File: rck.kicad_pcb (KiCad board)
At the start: 2 copper layers, 142.3 x 183.9 mm, 40 parts, among them J01 Conn_02x22_Row_Letter_Last, J02 Conn_02x22_Row_Letter_Last, J03 Conn_02x22_Row_Letter_Last, J04 Conn_02x22_Row_Letter_Last

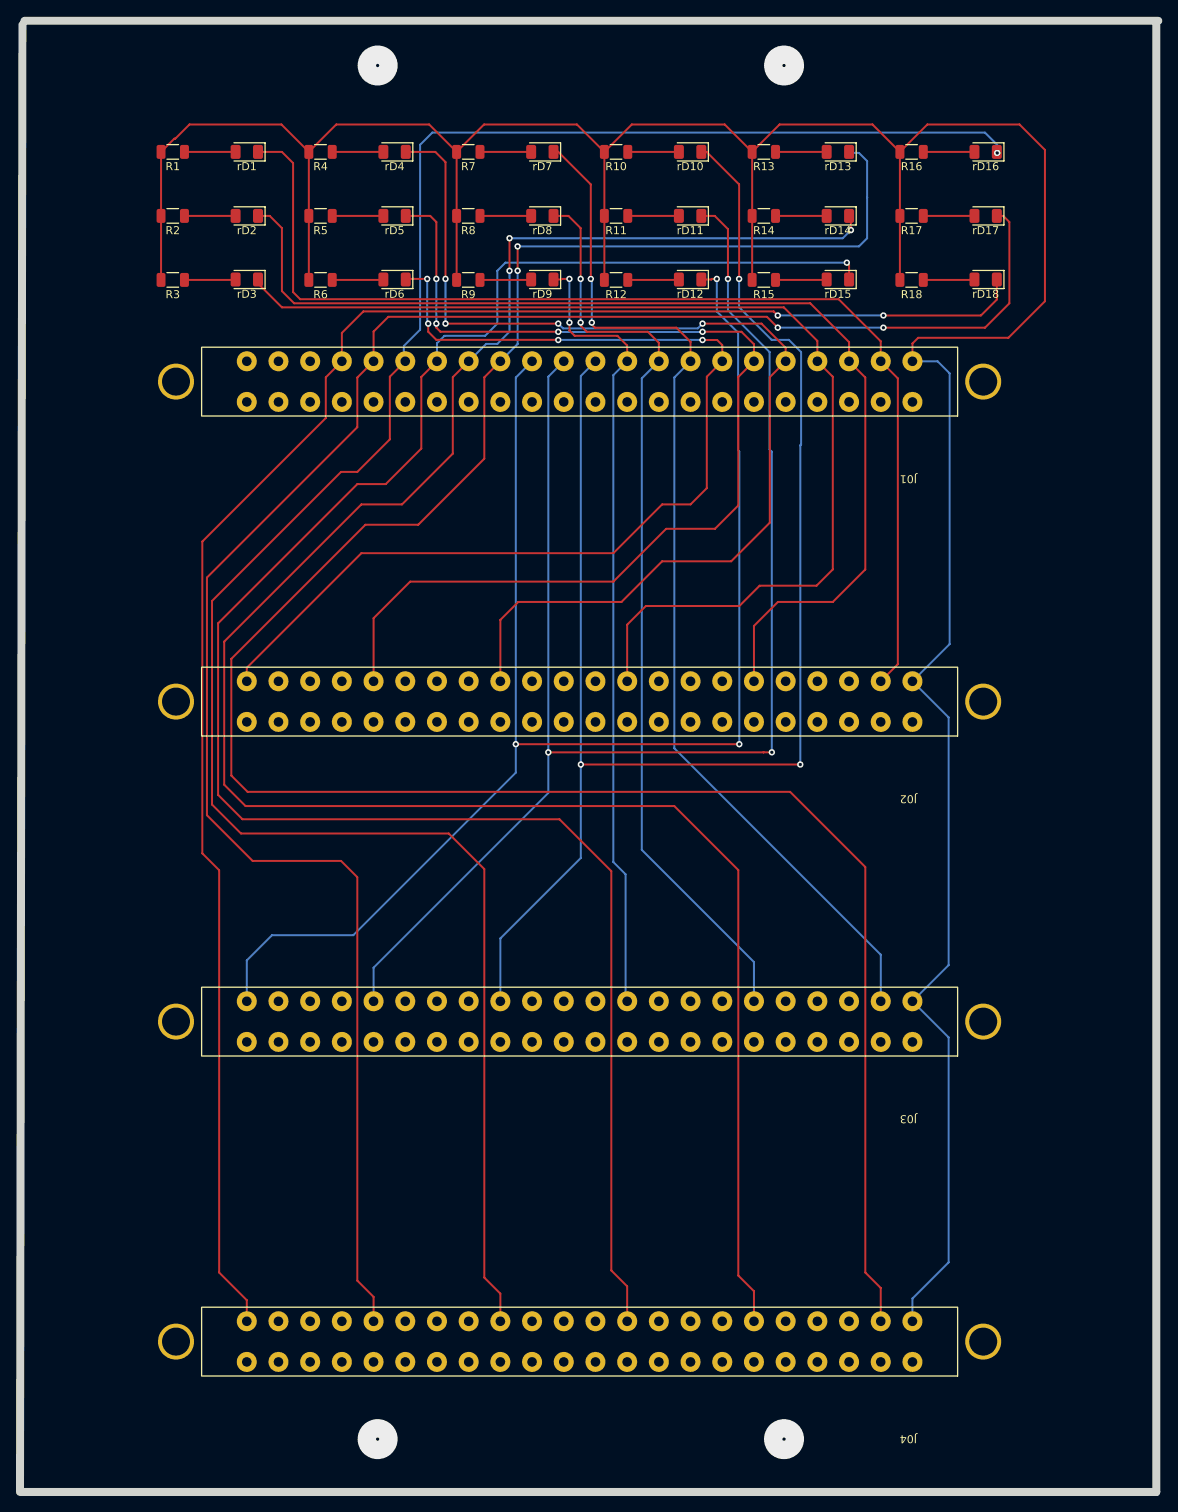
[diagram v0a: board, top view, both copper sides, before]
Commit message: V1.0Rack
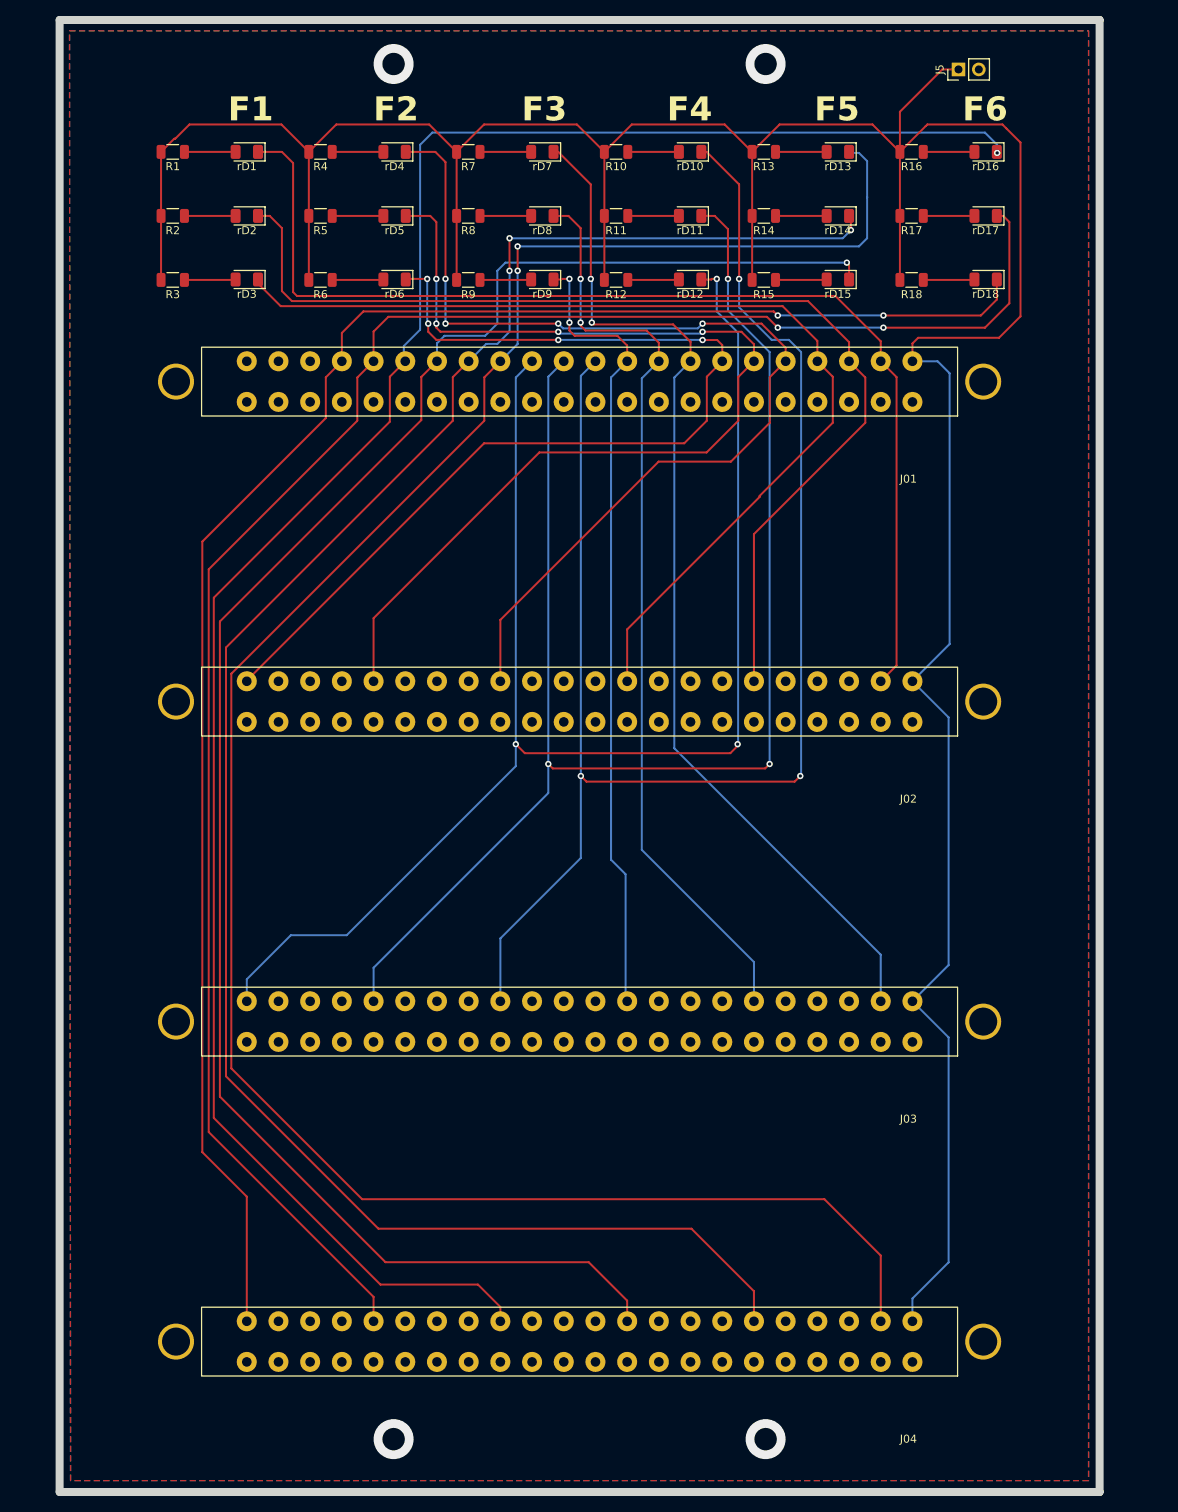
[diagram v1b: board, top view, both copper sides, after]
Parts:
- added J5: Conn_01x02_Pin, Connector_PinHeader_2.54mm:PinHeader_1x02_P2.54mm_Vertical, F.Cu at (148.8, 18.7)
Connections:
- J01 pad 22a: unconnected-(J01-Pin_22a-Pad22a) -> GND
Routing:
- net Net-(J01-Pin_15a): track 257.7 -> 246.1 mm
- net Net-(J01-Pin_4a): track 138.4 -> 127.4 mm
- net Net-(J01-Pin_16a): track 241.7 -> 231.1 mm
- net VCC: track 396.5 -> 406.6 mm
- net Net-(J01-Pin_14a): track 282.7 -> 272.9 mm
- net Net-(J01-Pin_17a): track 263.7 -> 254.3 mm
- net Net-(J01-Pin_5a): track 139.0 -> 131.7 mm
- net Net-(J01-Pin_18a): track 241.5 -> 234.9 mm
- net Net-(J01-Pin_6a): track 138.2 -> 132.2 mm
- net Net-(J01-Pin_7a): track 133.5 -> 127.6 mm
- net Net-(J01-Pin_3a): track 138.1 -> 134.0 mm
- net Net-(J01-Pin_11a): track 195.8 -> 197.8 mm
- net Net-(J01-Pin_12a): track 189.5 -> 191.0 mm
- net Net-(J01-Pin_13a): track 190.0 -> 189.0 mm
- added copper zone on B.Cu, net GND
- added copper zone on F.Cu, net GND
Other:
- board size 142.3 x 183.9 mm -> 130 x 184 mm
- board text added: "F1"
- board text added: "F2"
- board text added: "F3"
- board text added: "F4"
- board text added: "F5"
- board text added: "F6"
